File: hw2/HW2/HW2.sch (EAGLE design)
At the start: 22 parts, among them J1 USB-MB-H

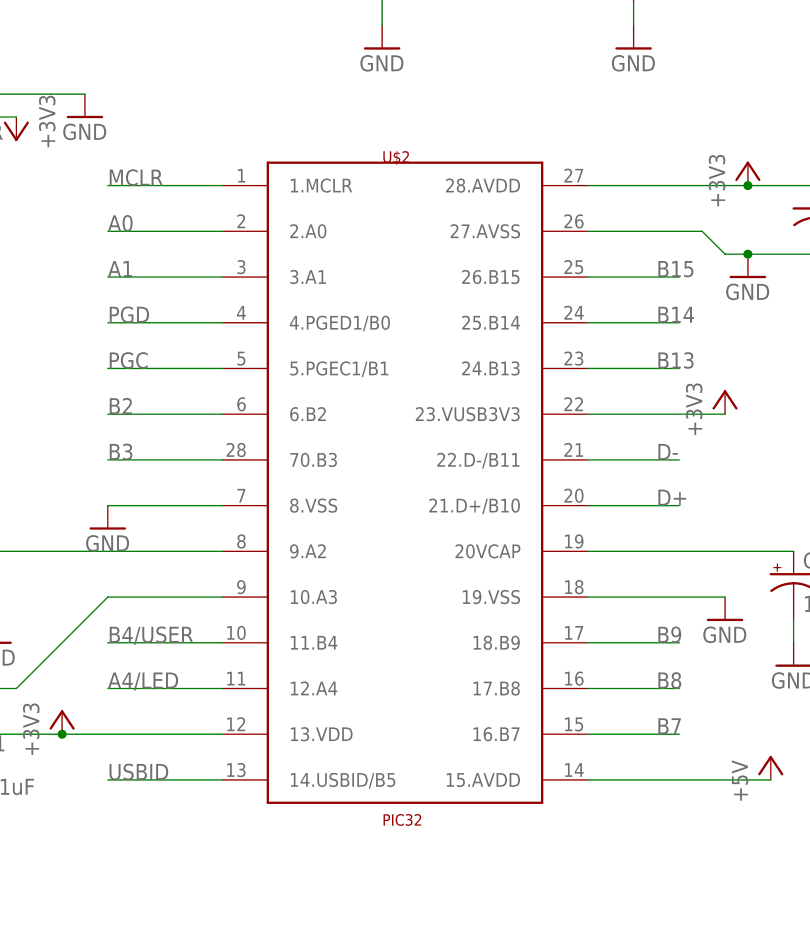
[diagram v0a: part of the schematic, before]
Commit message: Working on .brd
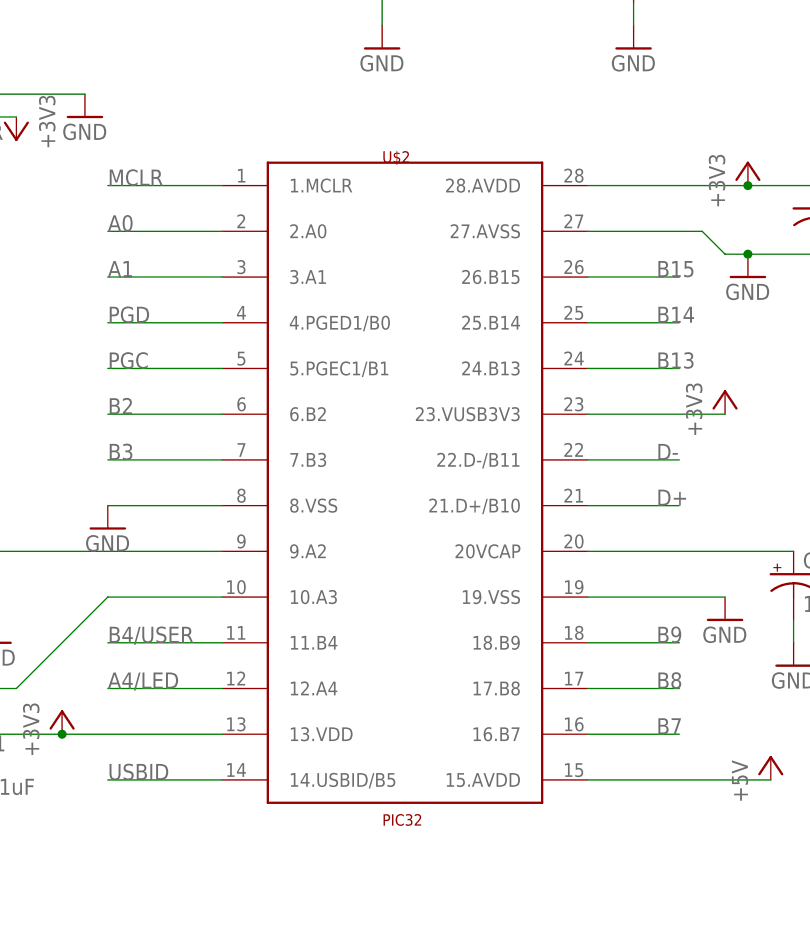
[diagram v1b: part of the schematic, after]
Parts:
- C5, C6: device HW2:CPOL-USETR2 -> HW2:CPOL-USB45181A
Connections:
- net B3: now also U$2.7.B3; no longer U$2.70.B3
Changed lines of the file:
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@@
 <part name="C3" library="HW2" deviceset="C-US" device="025-024X044" value="0.1uF"/>
 <part name="C4" library="HW2" deviceset="C-US" device="025-024X044" value="0.1uF"/>
-<part name="C5" library="HW2" deviceset="CPOL-US" device="ETR2" value="10uF"/>
-<part name="C6" library="HW2" deviceset="CPOL-US" device="ETR2" value="10uF"/>
+<part name="C5" library="HW2" deviceset="CPOL-US" device="B45181A" value="10uF"/>
+<part name="C6" library="HW2" deviceset="CPOL-US" device="B45181A" value="10uF"/>
 <part name="LED1" library="HW2" deviceset="LED" device="3MM" value="red"/>
 <part name="LED2" library="HW2" deviceset="LED" device="3MM" value="green"/>
@@
 <net name="B3" class="0">
 <segment>
-<pinref part="U$2" gate="G$1" pin="70.B3"/>
+<pinref part="U$2" gate="G$1" pin="7.B3"/>
 <wire x1="-20.32" y1="0" x2="-33.02" y2="0" width="0.1524" layer="91"/>
 <label x="-33.02" y="0" size="1.778" layer="95"/>
